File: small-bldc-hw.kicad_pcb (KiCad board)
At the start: 4 copper layers, 65 x 22.4 mm, 98 parts, among them J1 More IO, J2 TEMP, J3 CONN_01X01, J4 CONN_01X01, J5 CONN_01X01, J6 CAN, J7 I2C, J8 CONN_01X01, J9 CONN_01X01, P2 SWD, Q1 BUK7K13-60E, Q2 BUK7K13-60E, Q3 BUK7K13-60E, U1 STM32F042C6T6, U2 AZ1117C, U3 DRV8301, U4 MCP2562-E/SN, Y1 16MHz

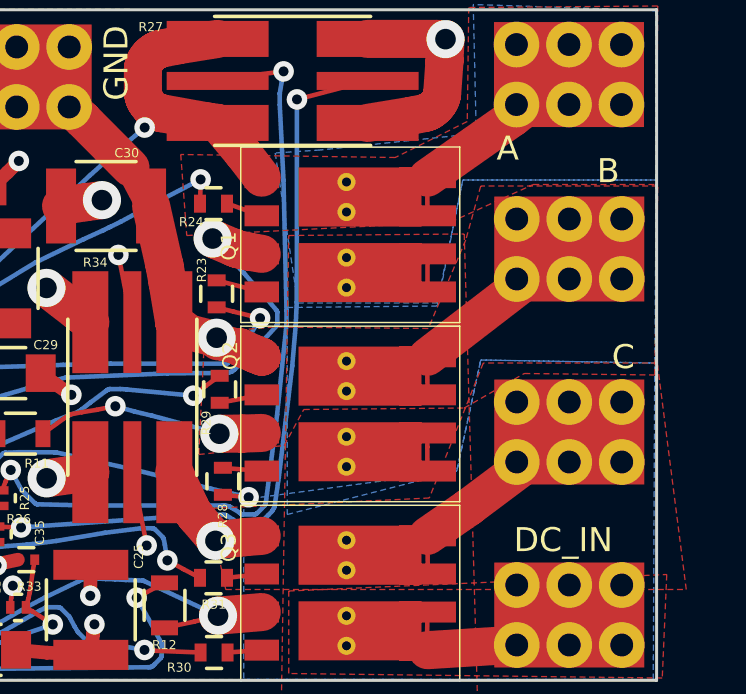
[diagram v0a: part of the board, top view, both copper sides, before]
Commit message: idk
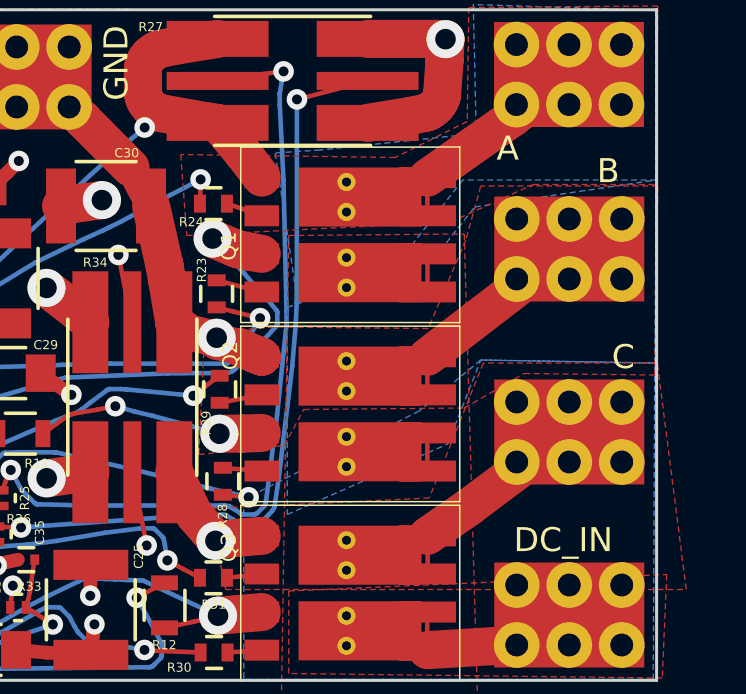
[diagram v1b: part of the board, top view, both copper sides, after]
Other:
- net class Default: clearance 0.1524 -> 0.153924
- net class smallpower: clearance 0.1524 -> 0.153924
- rule trace_clearance: 0.1524 -> 0.153924
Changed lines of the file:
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@@
   (page A4)
   (layers
-    (0 F.Cu signal)
-    (1 In1.Cu signal hide)
+    (0 F.Cu signal hide)
+    (1 In1.Cu signal)
     (2 In2.Cu signal hide)
-    (31 B.Cu signal hide)
+    (31 B.Cu signal)
     (35 F.Paste user)
     (36 B.SilkS user)
@@
   (setup
     (last_trace_width 0.1524)
-    (trace_clearance 0.1524)
+    (trace_clearance 0.153924)
     (zone_clearance 0.508)
     (zone_45_only no)
@@
   (net 89 /CAN_TX)
   (net_class Default "This is the default net class."
-    (clearance 0.1524)
+    (clearance 0.153924)
     (trace_width 0.1524)
     (via_dia 0.6858)
@@
   )
   (net_class smallpower ""
-    (clearance 0.1524)
+    (clearance 0.153924)
     (trace_width 0.4572)
     (via_dia 0.6858)
@@
       (pts
         (xy 184.9 89.75) (xy 178.8 89.55) (xy 178.9 93.85) (xy 173.7 94.4) (xy 172.2 94.5)
-        (xy 172.95 99.5) (xy 177.6 99.5) (xy 178.45 95.4) (xy 184.9 95.4)
+        (xy 172.95 99.5) (xy 177.7 97.75) (xy 178.85 96.3) (xy 184.9 95.4)
       )
     )
@@
     (polygon
       (pts
-        (xy 184.9 95.4) (xy 178.45 95.4) (xy 177.6 99.6) (xy 172.6 99.65) (xy 172.6 106.55)
-        (xy 178.25 105.1) (xy 179.05 101.4) (xy 184.85 101.5) (xy 184.9 95.45)
+        (xy 184.9 95.4) (xy 178.45 95.4) (xy 176.1 98.4) (xy 172.6 99.65) (xy 172.6 106.55)
+        (xy 177.95 104.2) (xy 179.05 101.4) (xy 184.85 101.5) (xy 184.9 95.45)
       )
     )
@@
       (pts
         (xy 171.15 106.05) (xy 171.15 112.05) (xy 184.8 112.05) (xy 184.85 101.5) (xy 179.05 101.4)
-        (xy 178.25 105.1)
+        (xy 177 103.1)
       )
     )

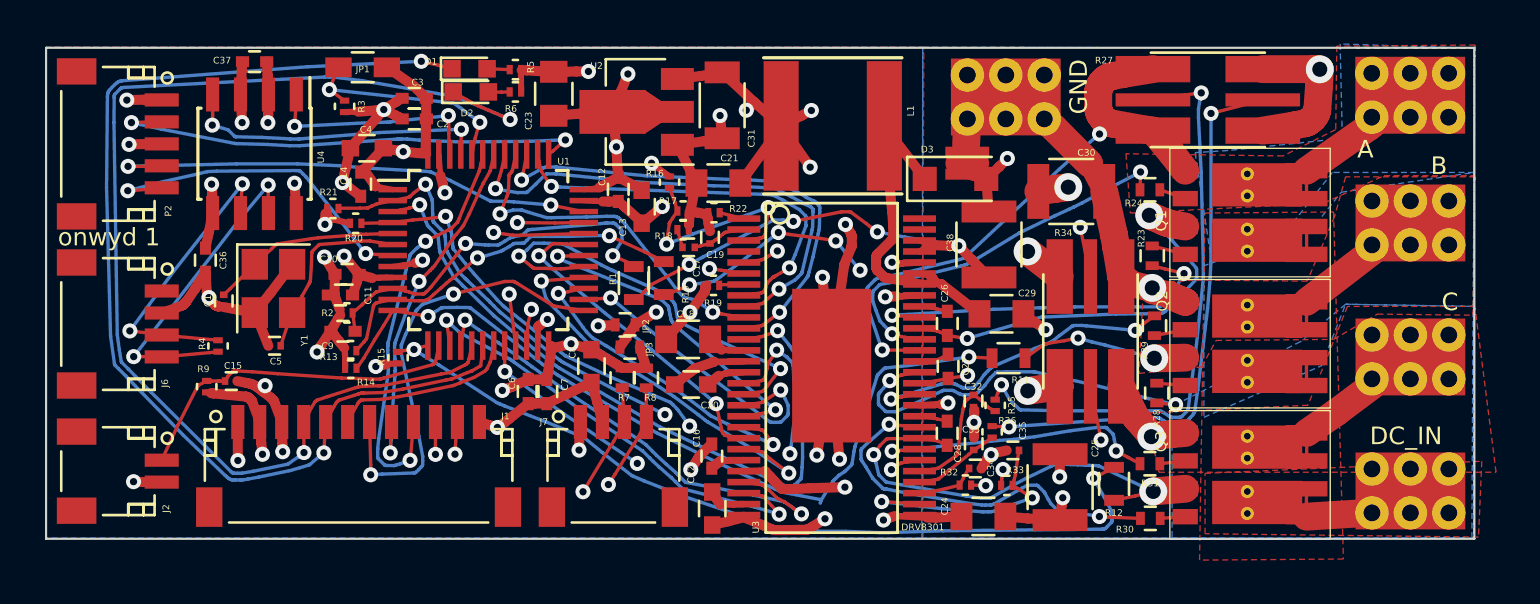
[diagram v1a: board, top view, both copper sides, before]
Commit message: I think something relating to planes was changed
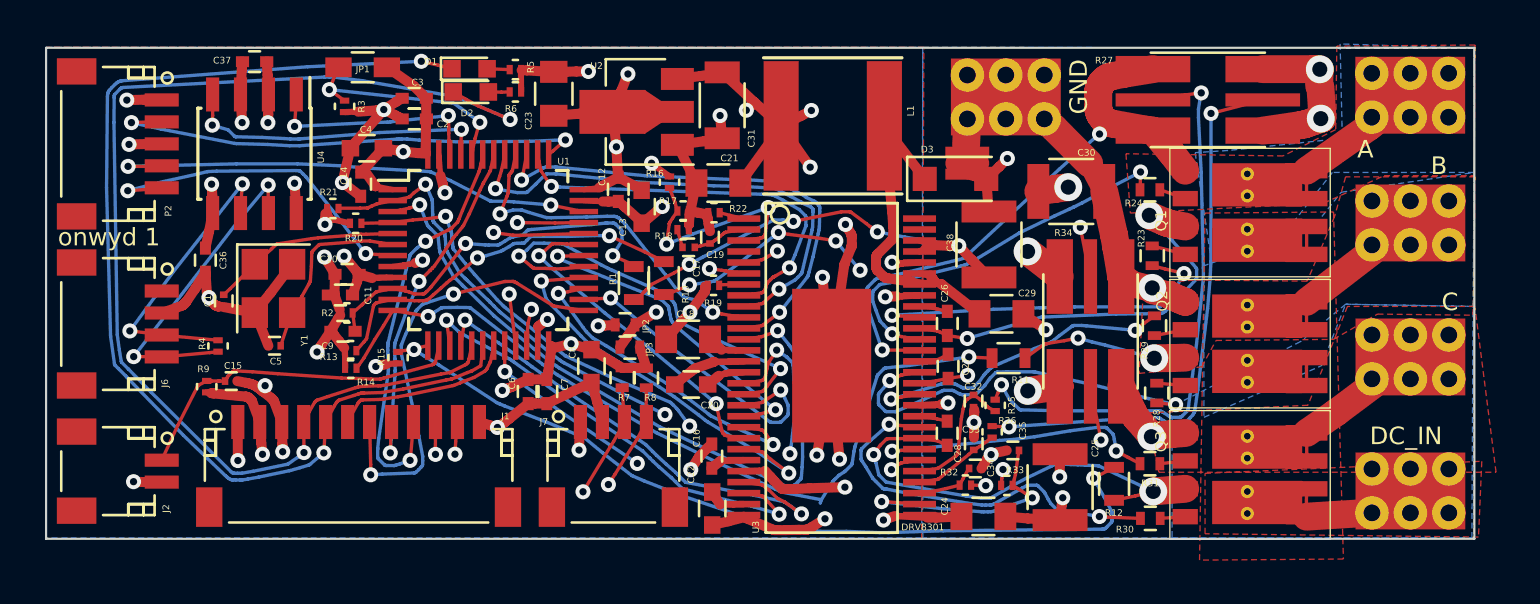
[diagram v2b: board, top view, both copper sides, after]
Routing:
- net GNDPWR: track 72.2 -> 72.5 mm, vias 4 -> 5
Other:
- net class Default: clearance 0.153924 -> 0.1524
- net class smallpower: clearance 0.153924 -> 0.1524
- rule trace_clearance: 0.153924 -> 0.1524
